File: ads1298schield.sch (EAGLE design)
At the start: 98 parts, among them IC1 MCP1640SOT23-6-HAND, U1 MCP73831, U2 LTC3440EMSPBF, X1 SDBMF, X2 USB-MICROB

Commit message: v0.4
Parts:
- added C26, C58, C59, C60, C64: 100nF, rcl:C-EUC1210
- added C61: 4.7uF, rcl:C-EUC1210
- added JP58: (no value), pinhead:PINHD-1X4
- added R27: 10k, resistor:R-EU_M1406
- added R28: 100k, resistor:R-EU_M1406
- added SW3: !RST, stm32f4stamp:SWITCH-B3U-1110-BOSS
- added U$3: STM32F411RE, micro-stm_v3:STM32F411RE
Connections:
- new net N$100: R28.1, SW3..1, U$3G$1.NRST
- new net N$87: C61.1, U$3G$1.VCAP1
- new net N$88: C26.2
- new net N$91: C58.2
- new net N$92: C26.1
- new net N$93: C58.1
- new net N$94: C59.1
- new net N$95: C60.1
- new net N$96: C59.2
- new net N$97: C60.2
- new net N$98: R27.2, U$3G$1.BOOT0
- new net N$99: C64.1, U$3G$1.VDDA
- new net SWCLK: U$3G$1.PA14
- new net SWDIO: U$3G$1.PA13
- net +3V3: now also JP58.1, R28.2, U$3G$2.VDD@1, U$3G$2.VDD@2, U$3G$2.VDD@3, U$3G$2.VDD@4
- net AGND: now also C61.2, C64.2, R27.1, SW3..2, U$3G$1.BOOT1/PB2, U$3G$1.VSSA, U$3G$2.VSS@1, U$3G$2.VSS@4
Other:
- note added: "SWD debugger header"

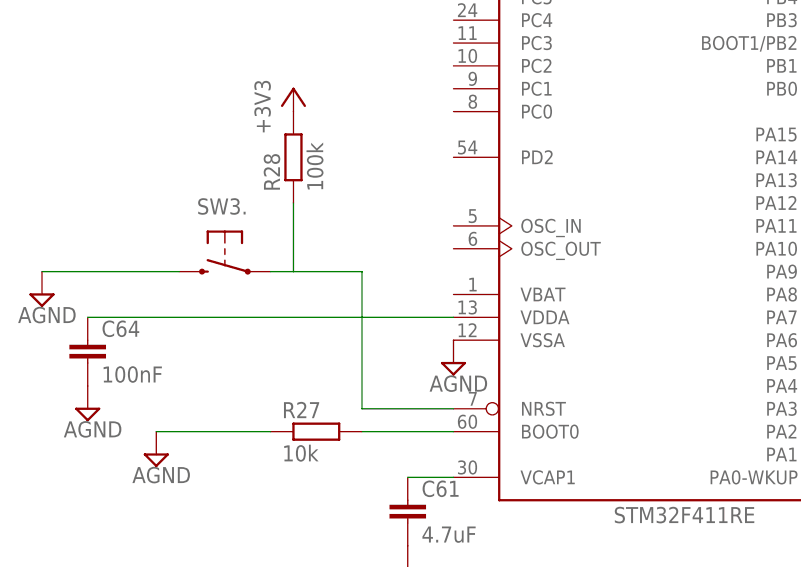
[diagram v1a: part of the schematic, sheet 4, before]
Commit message: v0.4
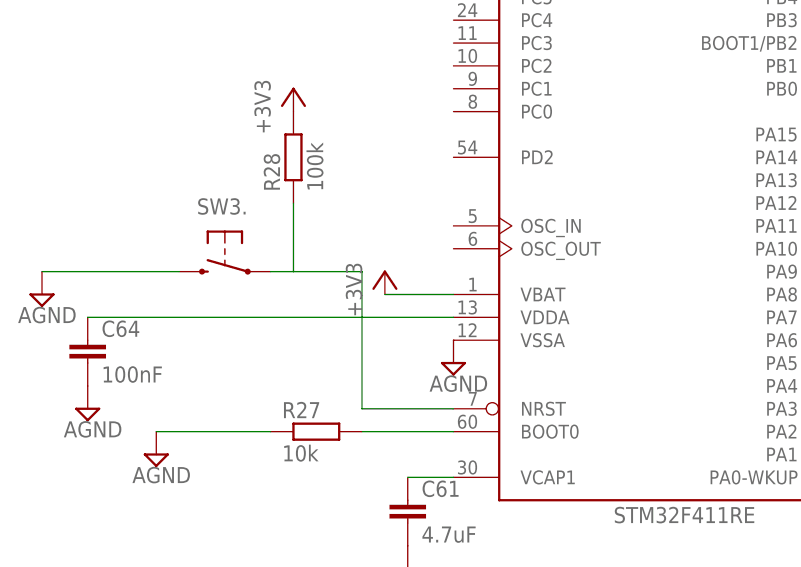
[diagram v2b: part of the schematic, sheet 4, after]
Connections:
- net +3V3: now also U$3G$1.VBAT
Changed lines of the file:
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@@
 <part name="+3V10" library="supply1" deviceset="+3V3" device=""/>
 <part name="SUPPLY38" library="supply2" deviceset="AGND" device=""/>
+<part name="+3V11" library="supply1" deviceset="+3V3" device=""/>
 </parts>
 <sheets>
@@
 <instance part="+3V10" gate="G$1" x="20.32" y="66.04"/>
 <instance part="SUPPLY38" gate="G$1" x="-7.62" y="43.18"/>
+<instance part="+3V11" gate="G$1" x="30.48" y="45.72"/>
 </instances>
 <busses>
@@
 <pinref part="+3V10" gate="G$1" pin="+3V3"/>
 </segment>
-</net>
+<segment>
+<pinref part="+3V11" gate="G$1" pin="+3V3"/>
+<pinref part="U$3" gate="G$1" pin="VBAT"/>
+<wire x1="30.48" y1="43.18" x2="38.1" y2="43.18" width="0.1524" layer="91"/>
+</segment>
+</net>
